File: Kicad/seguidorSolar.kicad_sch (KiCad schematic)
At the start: 15 parts, among them J1 Bateria, J2 Servo_1, J3 Servo_2, U1 ATtiny85V-10P, U2 AMS1117-5.0

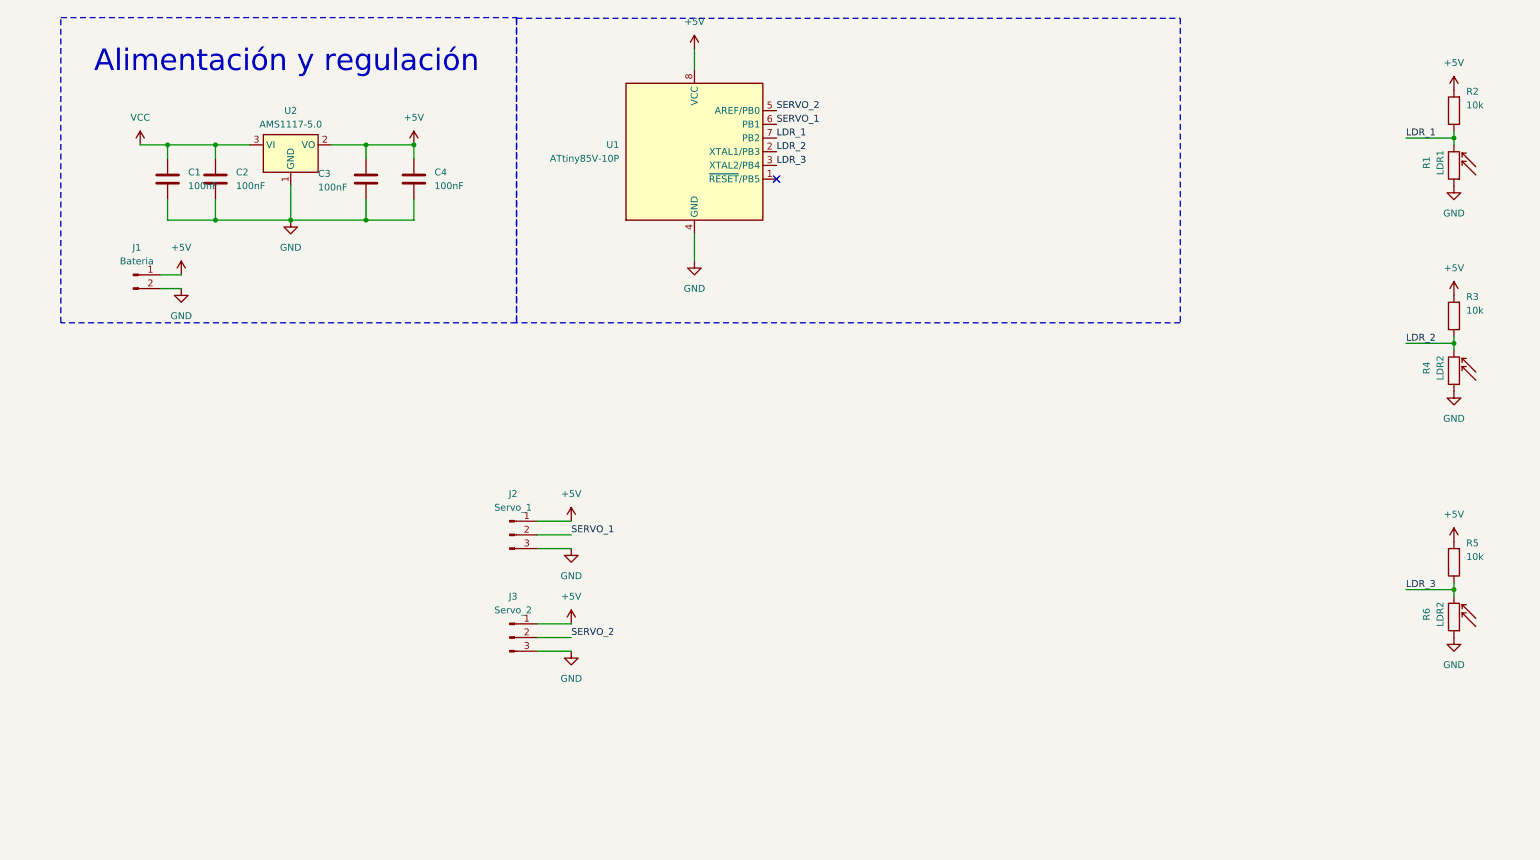
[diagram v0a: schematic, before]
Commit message: Add files via upload
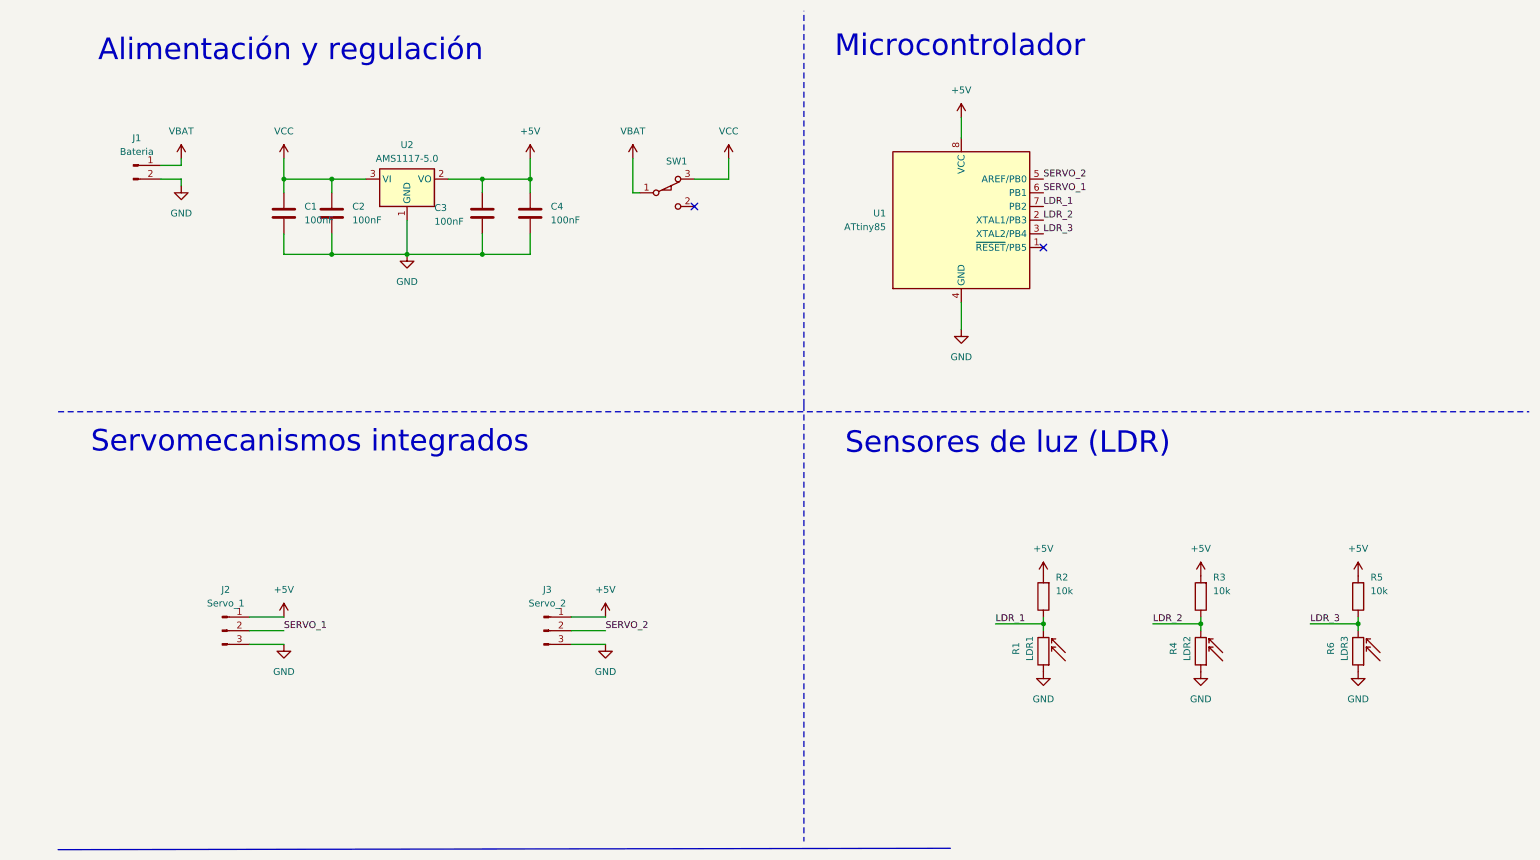
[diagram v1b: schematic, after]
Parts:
- added SW1: SW_SPDT_XKB_DMx-xxxx-1, Connector_PinHeader_2.54mm:PinHeader_1x03_P2.54mm_Vertical, symbol Switch:SW_SPDT_XKB_DMx-xxxx-1
- R6: value LDR2 -> LDR3
- U1: value ATtiny85V-10P -> ATtiny85
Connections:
- net +5V: no longer J1.1 (Pin_1)
- net VCC: now also SW1.3 (C)
- new net VBAT: J1.1 (Pin_1), SW1.1 (A)
- no-connect marks 1 -> 2
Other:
- note added: "Microcontrolador"
- note added: "Sensores de luz (LDR)"
- note added: "Servomecanismos integrados"
- moved on the sheet: C1, C2, C3, C4, J1, J2, J3, R1, R2, R3, R4, R5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
